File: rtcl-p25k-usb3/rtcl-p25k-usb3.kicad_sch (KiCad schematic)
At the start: 58 parts, among them J1 ZX360D-B-10P(30), J10 SSQ-106-02-F-D-RA, J2 0525592253, J3 BTB-DF40C-60DS-0.4V(51), J4 DF40C-60DS-0.4V(51), J5 JTAG, U12 TPS22917DBV, U2 TPD4E05U06DQA, U3 USBLC6-2P6, U4 FT601Q, X1 30MHz

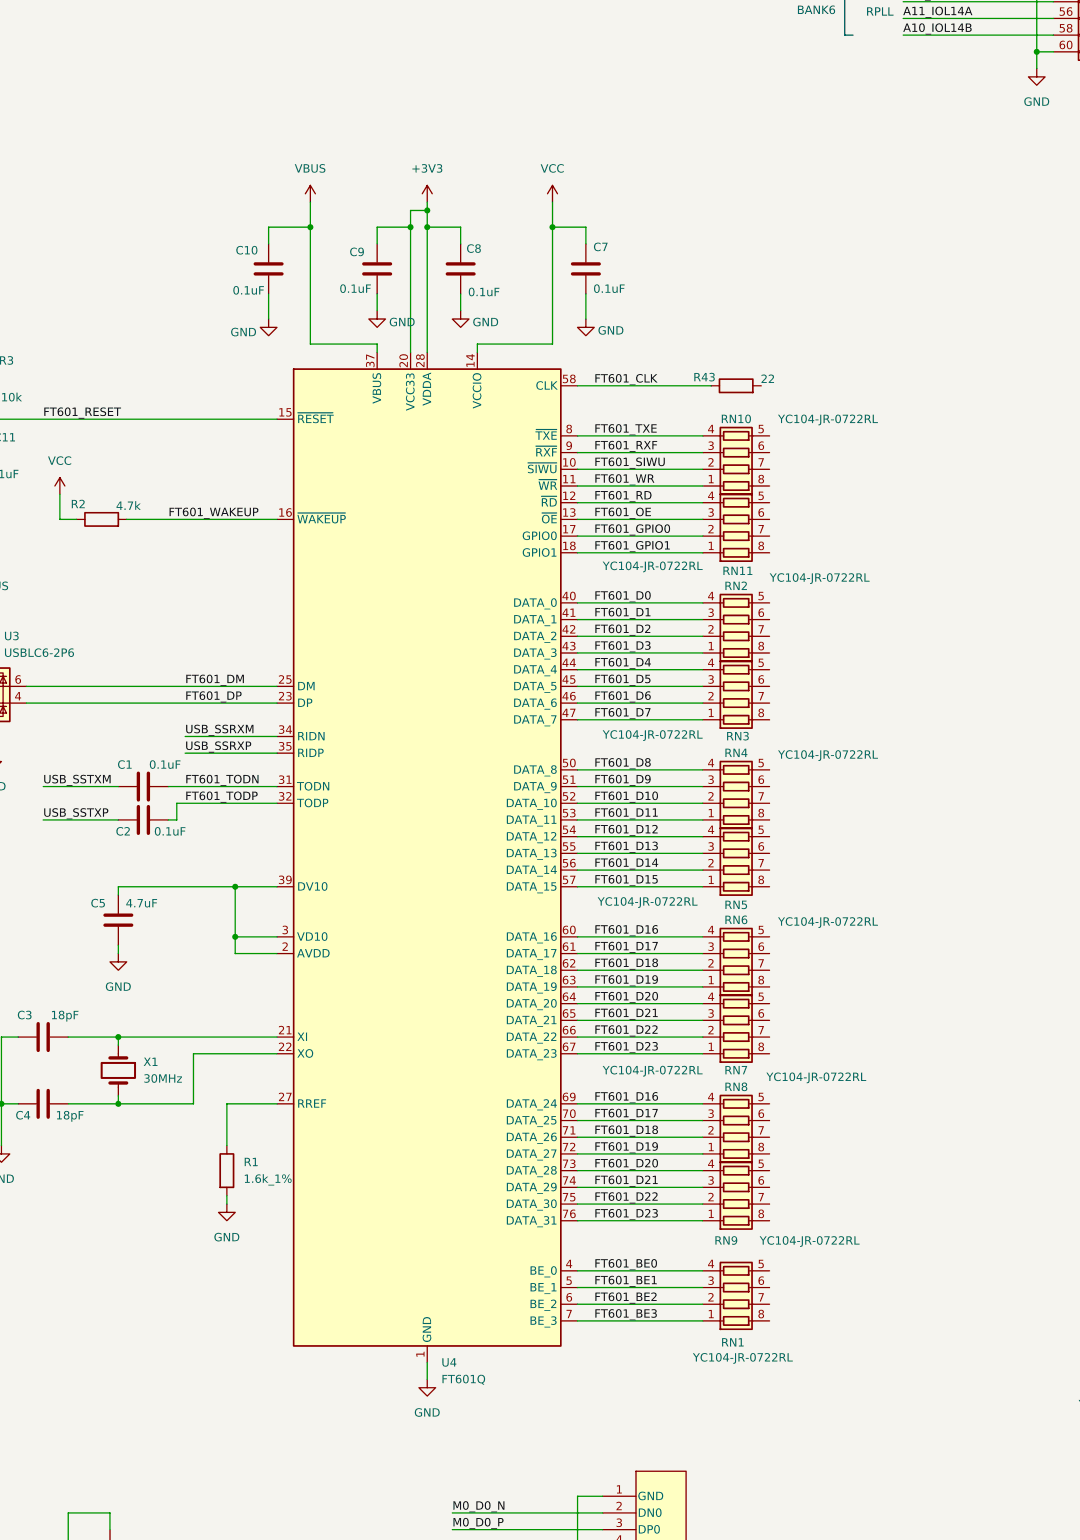
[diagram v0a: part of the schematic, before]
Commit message: WIP
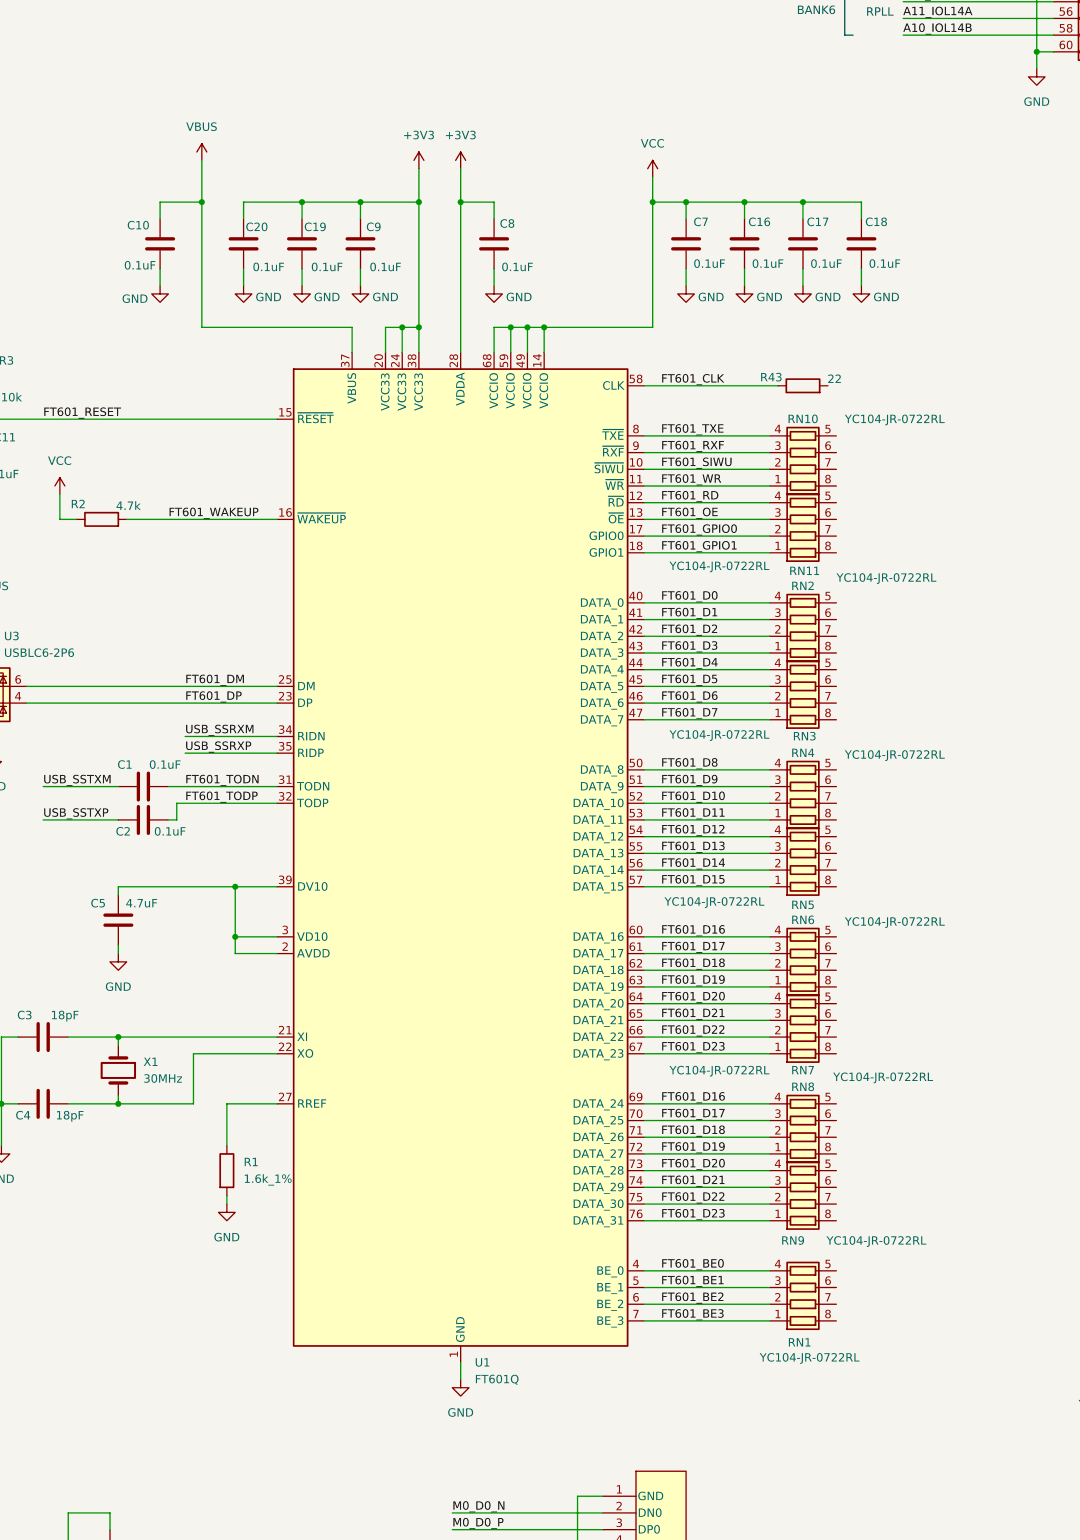
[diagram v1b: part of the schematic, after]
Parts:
- added C16, C17, C18, C19, C20: 0.1uF, Capacitor_SMD:C_0402_1005Metric, symbol Device:C
- J5: footprint Connector_PinHeader_2.54mm:PinHeader_1x08_P2.54mm_Vertical -> Connector_PinHeader_2.54mm:PinHeader_1x06_P2.54mm_Vertical
- renumbered U4 to U1
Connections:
- net +3V3: now also C19.2, C20.2
- net GND: now also C16.1, C17.1, C18.1, C19.1, C20.1
- net VCC: now also C16.2, C17.2, C18.2
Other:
- moved on the sheet: C10, C7, C8, C9, R43, RN1, RN10, RN11, RN2, RN3, RN4, RN5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
